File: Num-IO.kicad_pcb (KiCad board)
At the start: 2 copper layers, 170.2 x 77.5 mm, 101 parts, among them J1 DB37_Female, J2 DB37_Male, J3 Conn_02x25_Odd_Even, J4 0826-1X1T-GH-F, U1 MAX14917AFM+, U10 LTC6820IUD, U11 LTC6820IUD, U12 LTC6820IUD, U2 MAX14917AFM+, U3 MAX14851AEE+, U4 MAX14917AFM+, U5 MAX31910AUI+, U6 MAX31910AUI+, U7 MAX31910AUI+, U8 MAX31910AUI+, U9 LTC6820IUD

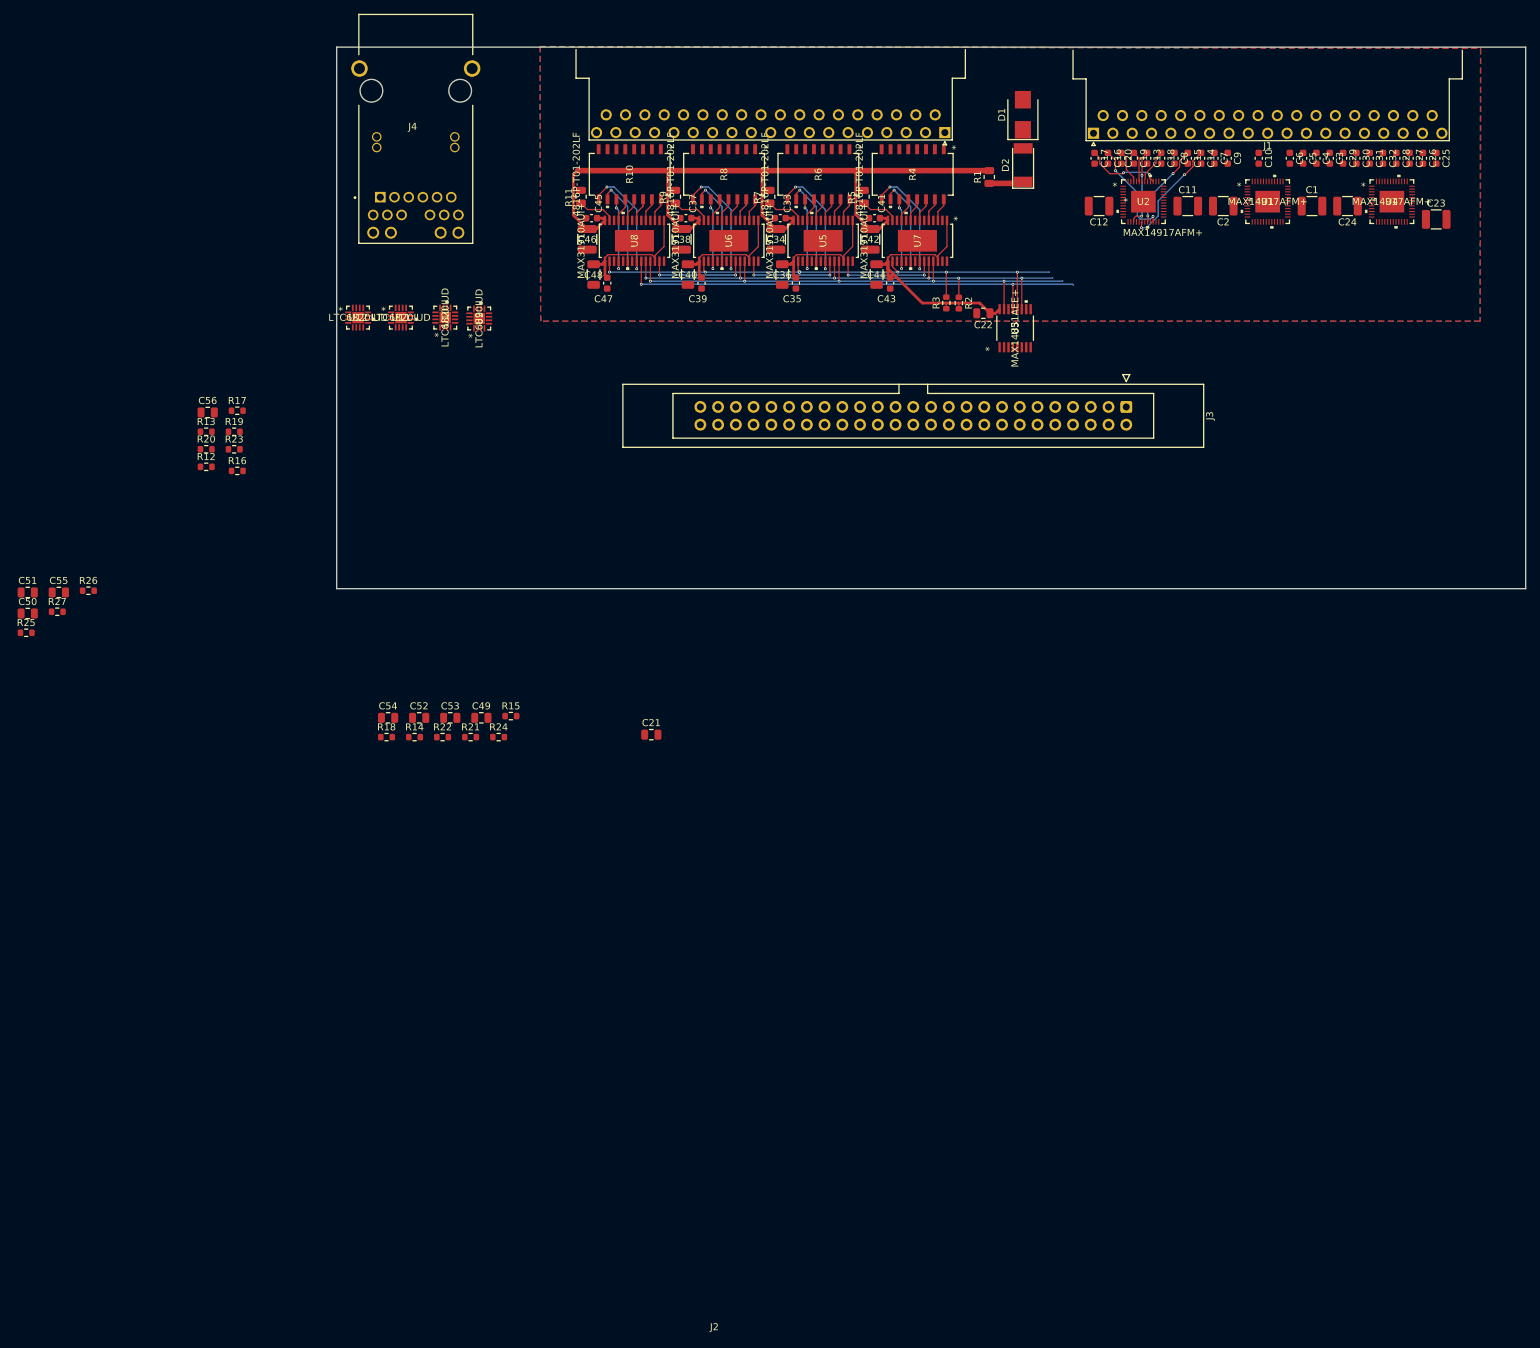
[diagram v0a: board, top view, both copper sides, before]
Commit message: fix DRC errors
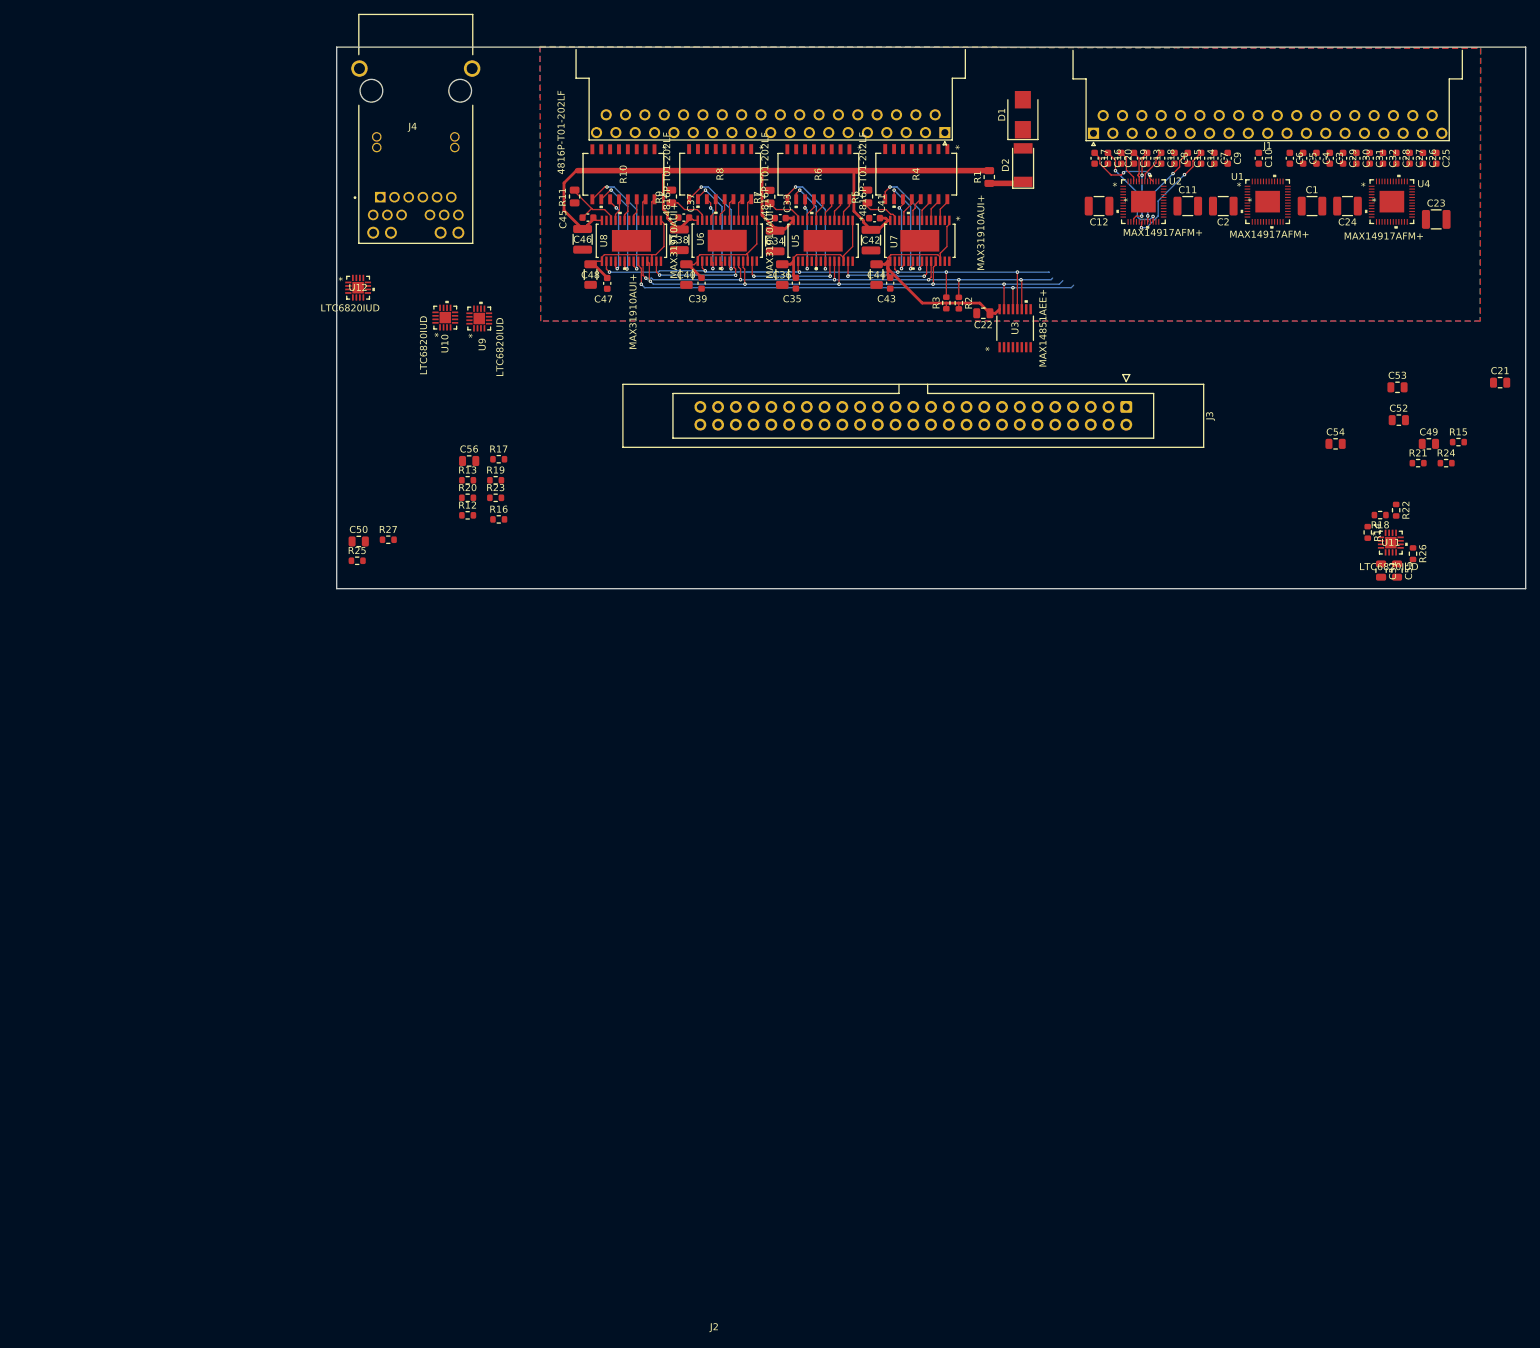
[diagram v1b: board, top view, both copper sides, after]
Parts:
- moved C51 193.7 mm to (209.3, 99.2), turned to -90 degrees
- moved C55 191.6 mm to (211.6, 99.2), turned to -90 degrees
- moved R26 189.7 mm to (213.8, 96.7), turned to -90 degrees
- moved C52 146.5 mm to (211.8, 77.6)
- moved R18 145.7 mm to (209.1, 91.2), turned to 180 degrees
- moved U11 145.3 mm to (210.7, 95.2)
- moved C53 143.6 mm to (211.6, 72.9)
- moved C49 141.2 mm to (216.1, 81.0)
- moved C54 141.2 mm to (202.8, 81.0)
- moved R15 141.2 mm to (220.3, 80.8)
- moved R21 141.2 mm to (214.6, 83.8)
- moved R24 141.2 mm to (218.6, 83.8)
- moved R22 140.3 mm to (211.4, 90.5), turned to -90 degrees
- moved R14 139.5 mm to (207.4, 93.7), turned to -90 degrees
- moved C21 131.5 mm to (226.3, 72.3)
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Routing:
- net GNDPWR: track 0.00 -> 9.33 mm
- net Net-(R11-Pad2): track 5.46 -> 0.00 mm
- net /CLK: track 74.5 -> 76.2 mm
- net /CS: track 75.2 -> 76.3 mm
- net Net-(R10-Pad9): track 17.4 -> 18.2 mm
- net Net-(R10-Pad10): track 14.8 -> 15.5 mm
- net /input channel 1-8/SDO: track 14.9 -> 15.5 mm
- net /input channel 17-24/5VOUT: track 19.2 -> 18.6 mm
- net Net-(R10-Pad11): track 11.1 -> 11.7 mm

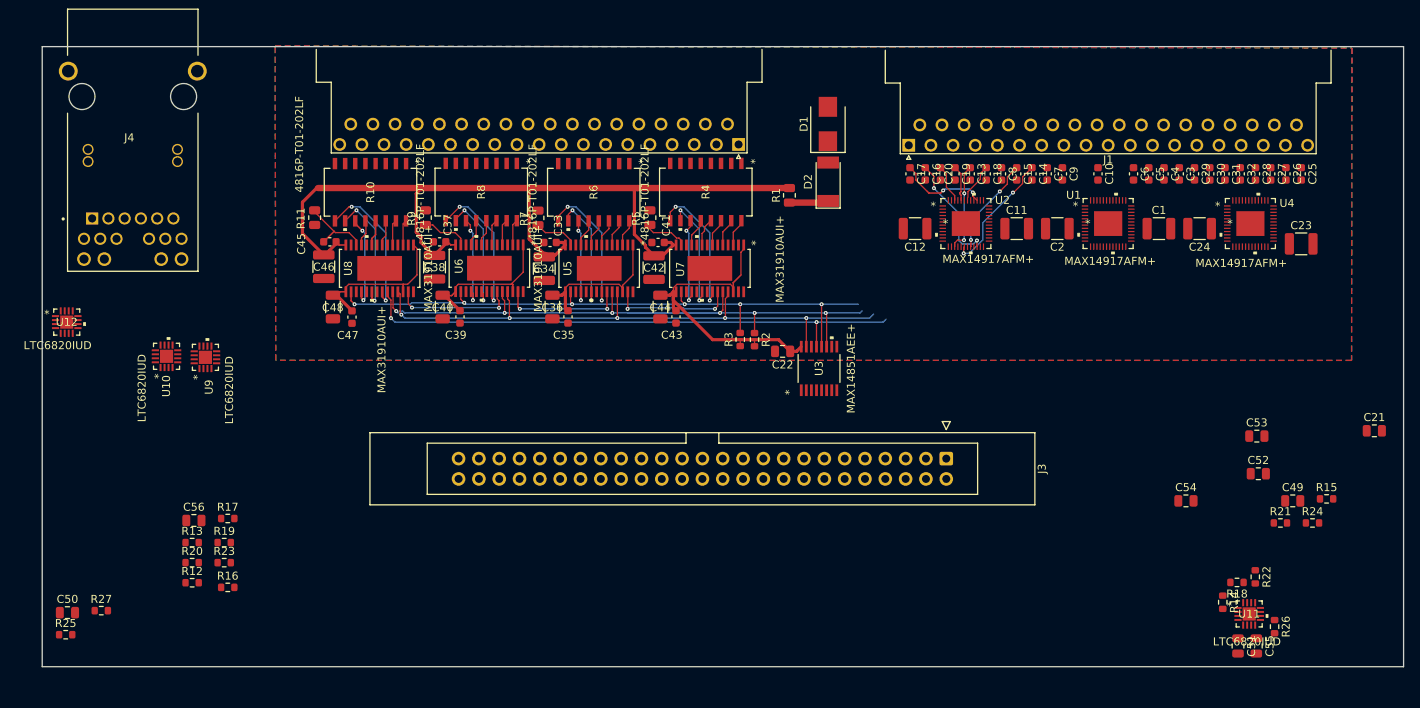
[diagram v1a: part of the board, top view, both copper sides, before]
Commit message: routing stuff
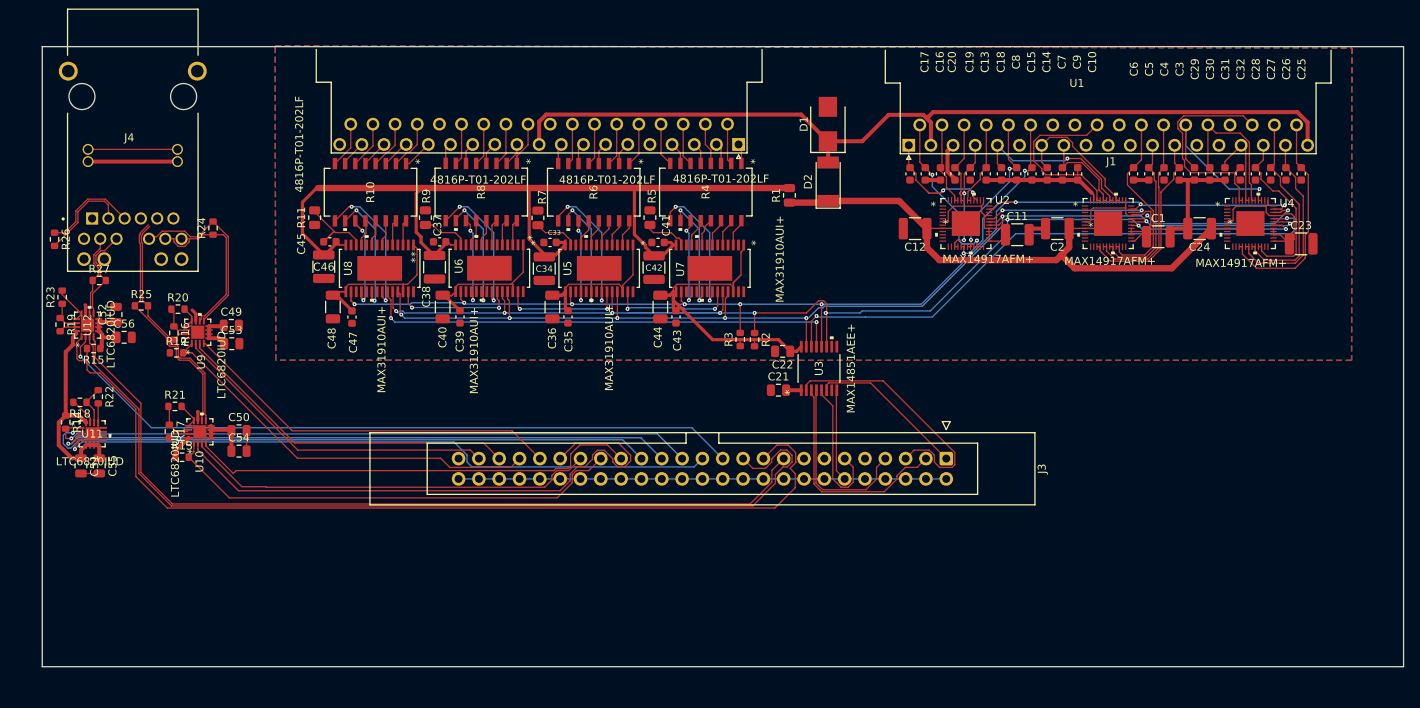
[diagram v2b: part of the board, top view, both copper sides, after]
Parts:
- C17: value 10nF -> 10nF->
- C6: value 10nF -> <-10nF
- moved R26 160.0 mm to (61.3, 48.3)
- moved R15 155.3 mm to (66.2, 62.0), turned to 180 degrees
- moved C51 146.4 mm to (64.6, 76.6)
- moved C55 146.4 mm to (66.9, 76.6)
- moved R14 146.4 mm to (62.7, 71.2)
- moved R18 146.4 mm to (64.5, 68.7)
- moved R22 146.4 mm to (66.8, 68.0)
- moved U11 146.4 mm to (66.0, 72.6)
- moved C52 144.2 mm to (69.0, 57.7), turned to 90 degrees
- moved R24 142.3 mm to (81.2, 46.9), turned to 90 degrees
- moved R21 138.9 mm to (76.4, 69.2)
- moved C49 134.5 mm to (83.4, 59.1)
- moved C53 128.6 mm to (83.5, 61.4)
- moved C54 118.5 mm to (84.4, 74.8)
- moved C21 74.7 mm to (151.8, 67.2)
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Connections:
- net Net-(J4-Pad10) renamed /RJ45 extension/TRD1-
- net Net-(J4-Pad11) renamed /RJ45 extension/TRD1+
- net Net-(J4-Pad2) renamed /RJ45 extension/TRD3-
- net Net-(J4-Pad3) renamed /RJ45 extension/TRD3+
- net Net-(J4-Pad4) renamed /RJ45 extension/TRD2+
- net Net-(J4-Pad5) renamed /RJ45 extension/TRD2-
- net Net-(J4-Pad8) renamed /RJ45 extension/TRD4+
- net Net-(J4-Pad9) renamed /RJ45 extension/TRD4-
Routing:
- net /FPGA Connector/SPI1.SDI: track 0.00 -> 118.9 mm
- net /FPGA Connector/SPI1.CLK: track 0.00 -> 114.9 mm
- net +24V: track 0.00 -> 112.2 mm
- net GNDD: track 0.00 -> 109.4 mm
- net /FPGA Connector/SPI1.*CS: track 0.00 -> 104.7 mm
- net /FPGA Connector/SPI1.SDO: track 0.00 -> 88.4 mm, vias 0 -> 1
- net /FPGA Connector/SPI2.*CS: track 0.00 -> 82.5 mm, vias 0 -> 1
- net /FPGA Connector/SPI2.SDI: track 0.00 -> 81.7 mm, vias 0 -> 1
- net /FPGA Connector/SPI2.CLK: track 0.00 -> 77.7 mm, vias 0 -> 1
- net /FPGA Connector/SPI2.SDO: track 0.00 -> 77.3 mm, vias 0 -> 1
- net OUTPWR: track 4.93 -> 79.4 mm
- net /SDI: track 0.00 -> 72.7 mm, vias 0 -> 2
- net /FPGA Connector/SPI3.SDO: track 0.00 -> 72.4 mm
- net /*FAULT: track 78.7 -> 145.5 mm, vias 6 -> 9
- net /CS: track 76.3 -> 143.0 mm, vias 6 -> 9
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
